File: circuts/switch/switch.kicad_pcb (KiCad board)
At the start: 2 copper layers, 45.4 x 50 mm, 16 parts, among them IC1 ATMEGA328P-TQFP32, IC2 SP3481CN, P1 Power, P2 UART, P3 RS485, P4 Relay GND, P5 Relay 5V, P6 BUTTONS, U1 LM78L05ACZ, U2 ULN2803L

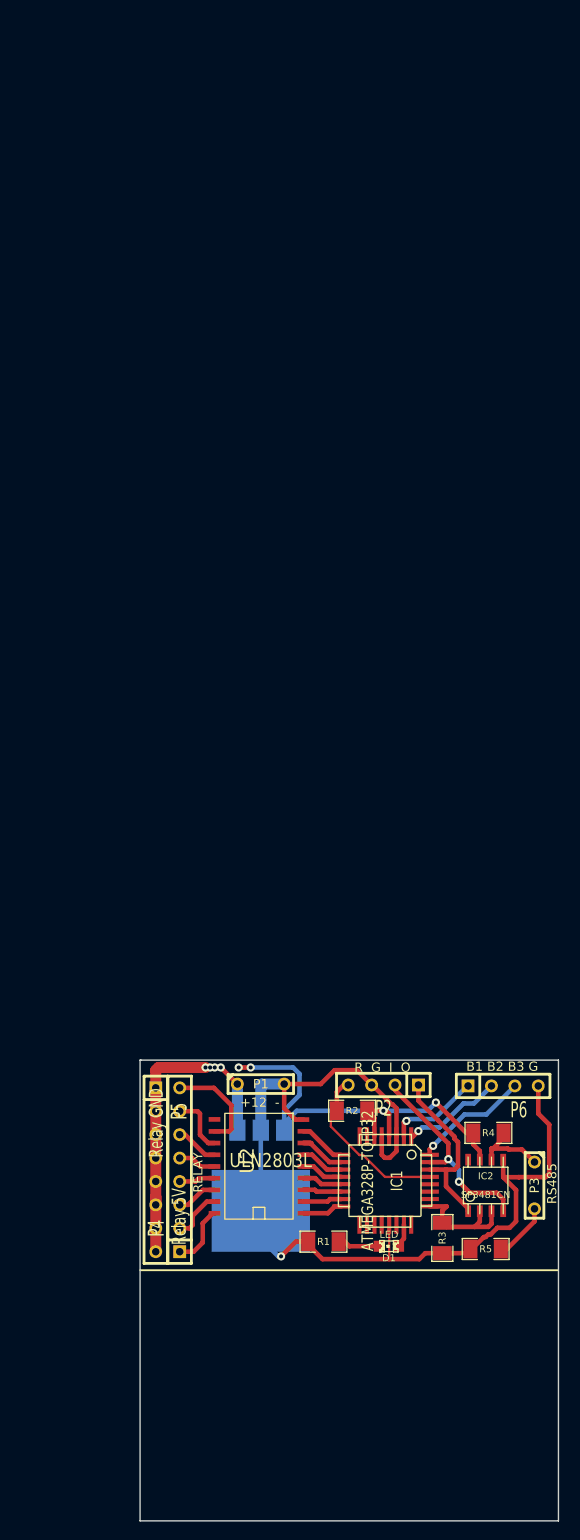
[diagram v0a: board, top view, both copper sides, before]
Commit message: Sended to prodaction
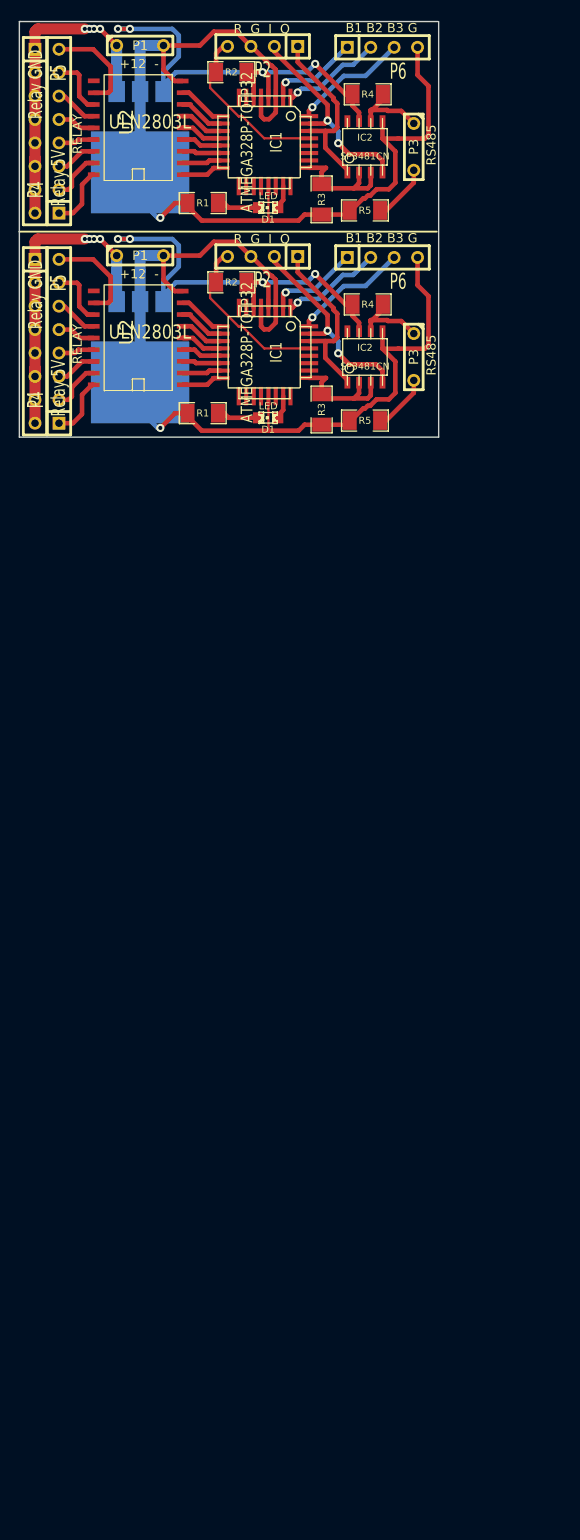
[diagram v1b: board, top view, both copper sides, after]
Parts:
- added D1: LED, LED-0805, F.Cu at (27.0, 43.0)
- added IC1: ATMEGA328P-TQFP32, TQFP32, F.Cu at (26.6, 35.9)
- added IC2: SP3481CN, so-8, F.Cu at (37.5, 36.4)
- added P1: Power, C2, F.Cu at (13.1, 25.4)
- added P2: UART, SIL-4, F.Cu at (26.4, 25.5)
- added P3: RS485, C2, F.Cu at (42.8, 36.4)
- added P4: Relay GND, SIL-8, F.Cu at (4.30, 34.7)
- added P5: Relay 5V, SIL-8, F.Cu at (1.70, 34.7)
- added P6: BUTTONS, SIL-4, F.Cu at (39.4, 25.6)
- added R1: 1K, SM1206, F.Cu at (19.9, 42.5)
- added R2: 1K, SM1206, F.Cu at (23.0, 28.3)
- added R3: 10K, SM1206, F.Cu at (32.8, 42.1)
- added R4: 560, SM1206, F.Cu at (37.8, 30.7)
- added R5: 560, SM1206, F.Cu at (37.5, 43.3)
- added U1: LM78L05ACZ, DPAK3, B.Cu at (13.1, 30.4)
- added U2: ULN2803L, SO18L, F.Cu at (12.9, 33.7)
- moved D1 113.5 mm to (27.0, 20.2)
- moved IC1 113.5 mm to (26.6, 13.1)
- moved IC2 113.5 mm to (37.5, 13.6)
- moved P1 113.5 mm to (13.1, 2.60)
- moved P2 113.5 mm to (26.4, 2.70)
- moved P3 113.5 mm to (42.8, 13.6)
- moved P6 113.5 mm to (39.4, 2.80)
- moved R1 113.5 mm to (19.9, 19.7)
- moved R2 113.5 mm to (23.0, 5.50)
- moved R3 113.5 mm to (32.8, 19.3)
- moved U1 113.5 mm to (13.1, 7.60)
- moved P4 113.5 mm to (4.30, 11.9)
- moved P5 113.5 mm to (1.70, 11.9)
- moved R4 113.5 mm to (37.8, 7.90)
- moved R5 113.5 mm to (37.5, 20.5)
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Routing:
- net GND: track 105.7 -> 211.4 mm, vias 1 -> 2
- net +5V: track 51.0 -> 102.0 mm, vias 4 -> 8
- net +12V: track 36.2 -> 72.5 mm, vias 5 -> 10
- net /DI: track 22.4 -> 44.8 mm, vias 2 -> 4
- net /DO: track 19.3 -> 38.6 mm
- net /Reset: track 18.0 -> 36.0 mm
- net /Dir: track 12.8 -> 25.6 mm
- net /But3: track 12.7 -> 25.4 mm, vias 1 -> 2
- net /But2: track 11.0 -> 22.0 mm, vias 1 -> 2
- net N-0000017: track 10.9 -> 21.8 mm
- net /But1: track 10.2 -> 20.3 mm, vias 1 -> 2
- net N-0000021: track 9.05 -> 18.1 mm
- net N-000009: track 6.73 -> 13.5 mm
- net N-0000013: track 6.55 -> 13.1 mm
- net N-0000020: track 6.25 -> 12.5 mm
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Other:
- board size 45.4 x 50 mm -> 45.5 x 45.1 mm
